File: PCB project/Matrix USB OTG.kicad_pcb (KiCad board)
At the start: 2 copper layers, 29.2 x 19.5 mm, 2 parts, among them J1 USB3150-30-130-A, J2 SSM-102-L-DV

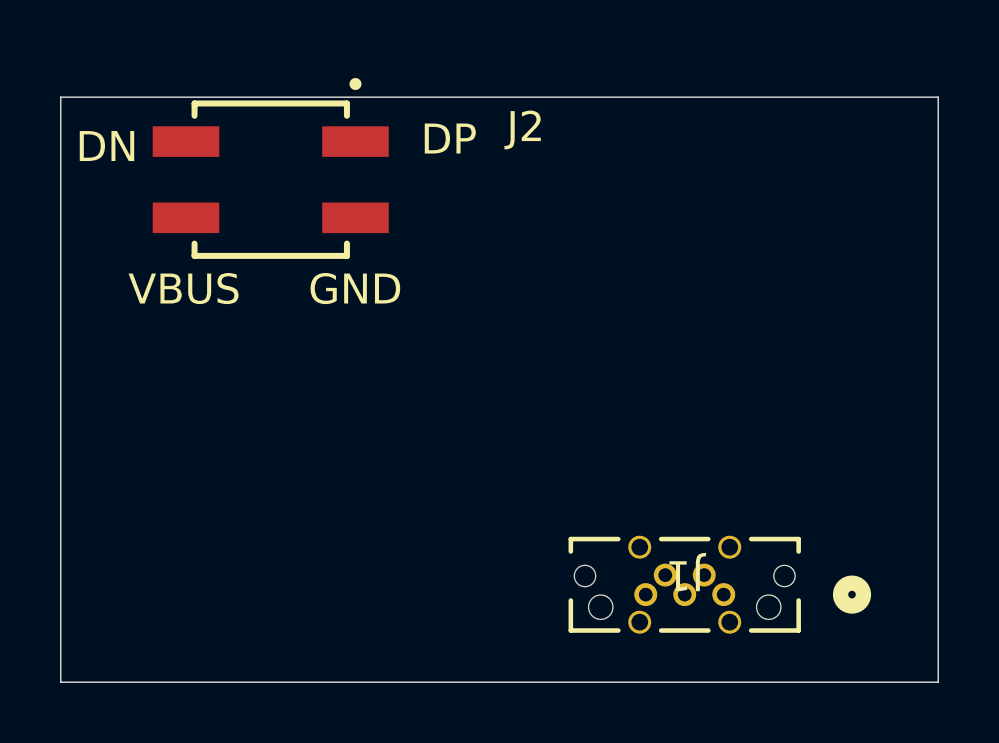
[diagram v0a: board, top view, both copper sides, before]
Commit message: Final shape before review
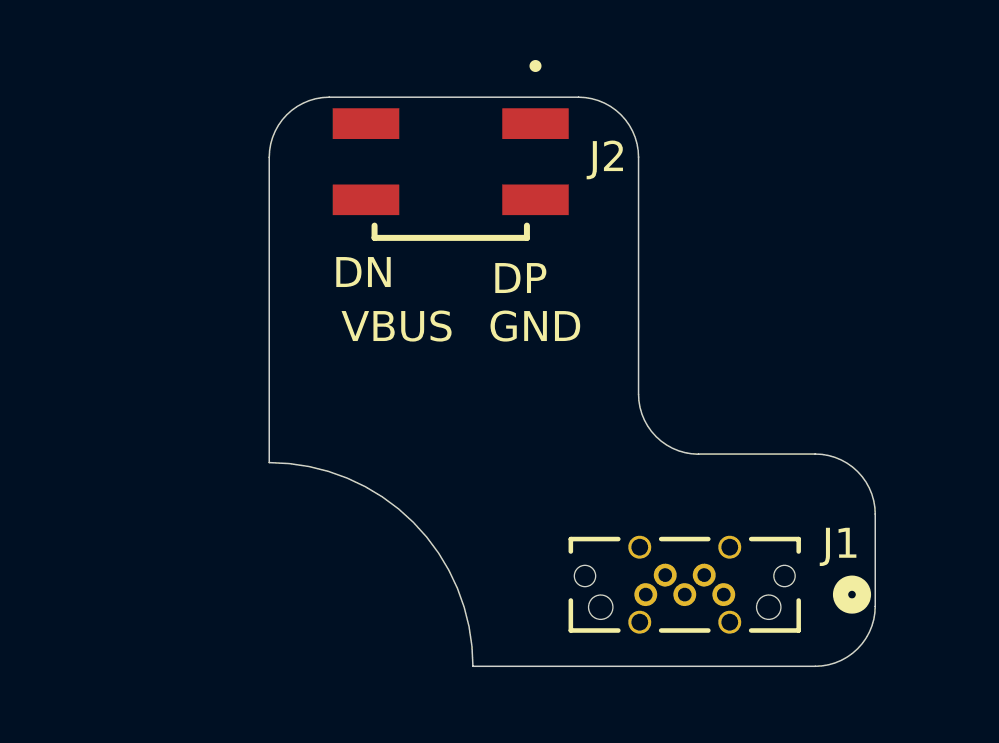
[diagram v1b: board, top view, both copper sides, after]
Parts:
- moved J2 6.03 mm to (113.7, 97.9)
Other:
- board size 29.2 x 19.5 mm -> 20.2 x 19 mm
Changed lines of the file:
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@@
 		(capping no)
 		(filling no)
-		(zone_defaults)
 		(pcbplotparams
 			(layerselection 0x00000000_00000000_55555555_5755f5ff)
@@
 	(footprint "Matrix-USB-OTG:SAMTEC_SSM-102-L-DV"
 		(layer "F.Cu")
-		(at 107.75 98.5 90)
+		(at 113.749999 97.899999 90)
 		(property "Reference" "J2"
-			(at 1.75 8.5 180)
+			(at 0.149999 5.240001 180)
 			(layer "F.SilkS")
 			(effects
@@
 		)
 		(property "Value" "SSM-102-L-DV"
-			(at 8.525 5.8 90)
+			(at -5.650001 -5.069999 90)
 			(layer "F.Fab")
 			(effects
@@
 		(sheetname "/")
 		(sheetfile "Matrix USB OTG.kicad_sch")
-		(units
-			(unit
-				(name "A")
-				(pins "01" "03" "02" "04")
-			)
-		)
 		(attr smd)
 		(duplicate_pad_numbers_are_jumpers no)
 		(fp_line
-			(start 2.54 -2.54)
-			(end 2.54 2.54)
-			(stroke
-				(width 0.2)
-				(type solid)
-			)
-			(layer "F.SilkS")
-		)
-		(fp_line
-			(start 2.13 -2.54)
-			(end 2.54 -2.54)
-			(stroke
-				(width 0.2)
-				(type solid)
-			)
-			(layer "F.SilkS")
-		)
-		(fp_line
 			(start -2.54 -2.54)
 			(end -2.13 -2.54)
-			(stroke
-				(width 0.2)
-				(type solid)
-			)
-			(layer "F.SilkS")
-		)
-		(fp_line
-			(start 2.13 2.54)
-			(end 2.54 2.54)
 			(stroke
 				(width 0.2)
@@
 		(tags "USB3150-30-130-A ")
 		(property "Reference" "J1"
-			(at 1.3 0.65 180)
+			(at -3.910001 1.690001 0)
 			(unlocked yes)
 			(layer "F.SilkS")
@@
 		)
 		(property "Value" "USB3150-30-130-A"
-			(at 1.3 0.65 180)
+			(at 3.959999 3.310001 0)
 			(unlocked yes)
 			(layer "F.Fab")
@@
 		)
 	)
-	(gr_rect
-		(start 100.75 95.75)
-		(end 130 115.25)
-		(stroke
-			(width 0.05)
-			(type default)
-		)
-		(fill no)
+	(gr_arc
+		(start 107.7 97.75)
+		(mid 108.285786 96.335786)
+		(end 109.7 95.75)
+		(stroke
+			(width 0.05)
+			(type default)
+		)
+		(layer "Edge.Cuts")
+	)
+	(gr_line
+		(start 107.7 107.93)
+		(end 107.7 97.75)
+		(stroke
+			(width 0.05)
+			(type default)
+		)
+		(layer "Edge.Cuts")
+	)
+	(gr_arc
+		(start 107.7 107.93)
+		(mid 112.501255 109.918745)
+		(end 114.49 114.72)
+		(stroke
+			(width 0.05)
+			(type default)
+		)
+		(layer "Edge.Cuts")
+	)
+	(gr_line
+		(start 109.7 95.75)
+		(end 118.01 95.75)
+		(stroke
+			(width 0.05)
+			(type default)
+		)
+		(layer "Edge.Cuts")
+	)
+	(gr_line
+		(start 114.49 114.72)
+		(end 125.9 114.72)
+		(stroke
+			(width 0.05)
+			(type default)
+		)
+		(layer "Edge.Cuts")
+	)
+	(gr_arc
+		(start 118.01 95.75)
+		(mid 119.424214 96.335786)
+		(end 120.01 97.75)
+		(stroke
+			(width 0.05)
+			(type default)
+		)
+		(layer "Edge.Cuts")
+	)
+	(gr_line
+		(start 120.01 97.74)
+		(end 120.01 105.65)
+		(stroke
+			(width 0.05)
+			(type default)
+		)
+		(layer "Edge.Cuts")
+	)
+	(gr_arc
+		(start 122.01 107.65)
+		(mid 120.595786 107.064214)
+		(end 120.01 105.65)
+		(stroke
+			(width 0.05)
+			(type default)
+		)
+		(layer "Edge.Cuts")
+	)
+	(gr_line
+		(start 125.9 107.644214)
+		(end 122.01 107.644214)
+		(stroke
+			(width 0.05)
+			(type default)
+		)
+		(layer "Edge.Cuts")
+	)
+	(gr_arc
+		(start 125.9 107.644214)
+		(mid 127.314214 108.23)
+		(end 127.9 109.644214)
+		(stroke
+			(width 0.05)
+			(type default)
+		)
+		(layer "Edge.Cuts")
+	)
+	(gr_line
+		(start 127.9 109.644214)
+		(end 127.9 112.72)
+		(stroke
+			(width 0.05)
+			(type default)
+		)
+		(layer "Edge.Cuts")
+	)
+	(gr_arc
+		(start 127.9 112.72)
+		(mid 127.314214 114.134214)
+		(end 125.9 114.72)
+		(stroke
+			(width 0.05)
+			(type default)
+		)
 		(layer "Edge.Cuts")
 	)
 	(gr_text "DN"
-		(at 101.25 98 0)
+		(at 109.8 102.2 0)
 		(layer "F.SilkS")
 		(effects
@@
 	)
 	(gr_text "VBUS"
-		(at 103 102.75 0)
+		(at 110.1 104 0)
 		(layer "F.SilkS")
 		(effects
@@
 	)
 	(gr_text "GND"
-		(at 109 102.75 0)
+		(at 115 104 0)
 		(layer "F.SilkS")
 		(effects
@@
 	)
 	(gr_text "DP"
-		(at 112.75 97.75 0)
+		(at 115.1 102.4 0)
 		(layer "F.SilkS")
 		(effects
